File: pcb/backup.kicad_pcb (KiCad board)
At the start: 2 copper layers, 47.6 x 63.5 mm, 44 parts, among them CON1 BARREL_JACK, IC1 ATMEGA168A-P, P1 CONN_02X02, P2 CONN_01X06, P3 CONN_01X07, P4 CONN_01X04, P5 CONN_01X07, SW1 SW_PUSH, U1 MAX6817, U2 LM7805CT, U3 MIC94090, Y1 Crystal

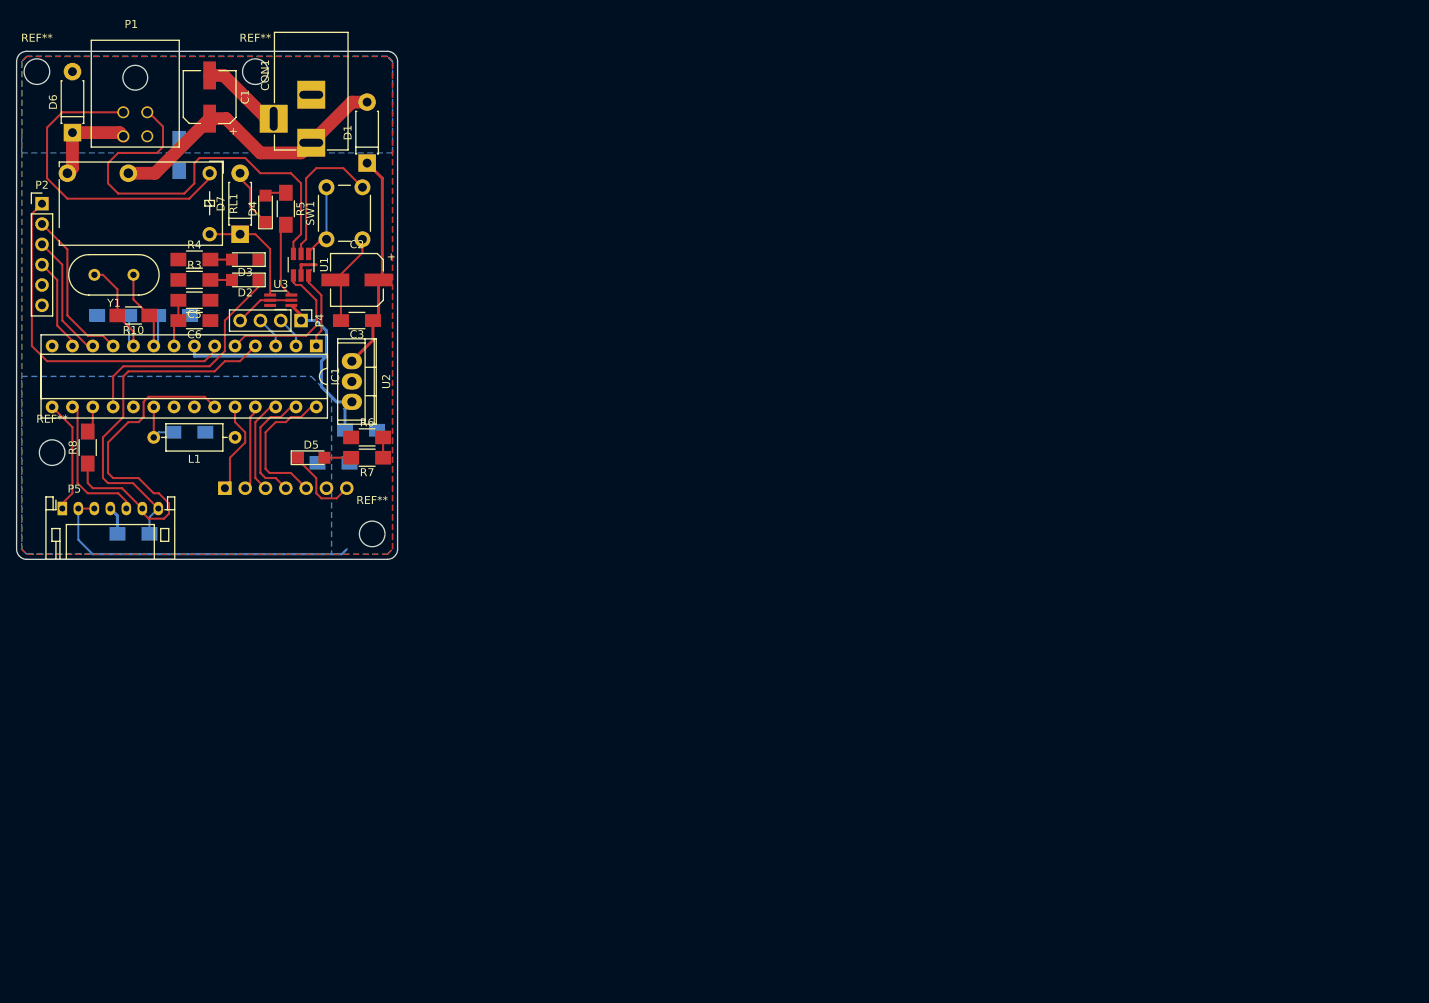
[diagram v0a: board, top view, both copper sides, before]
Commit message: wip
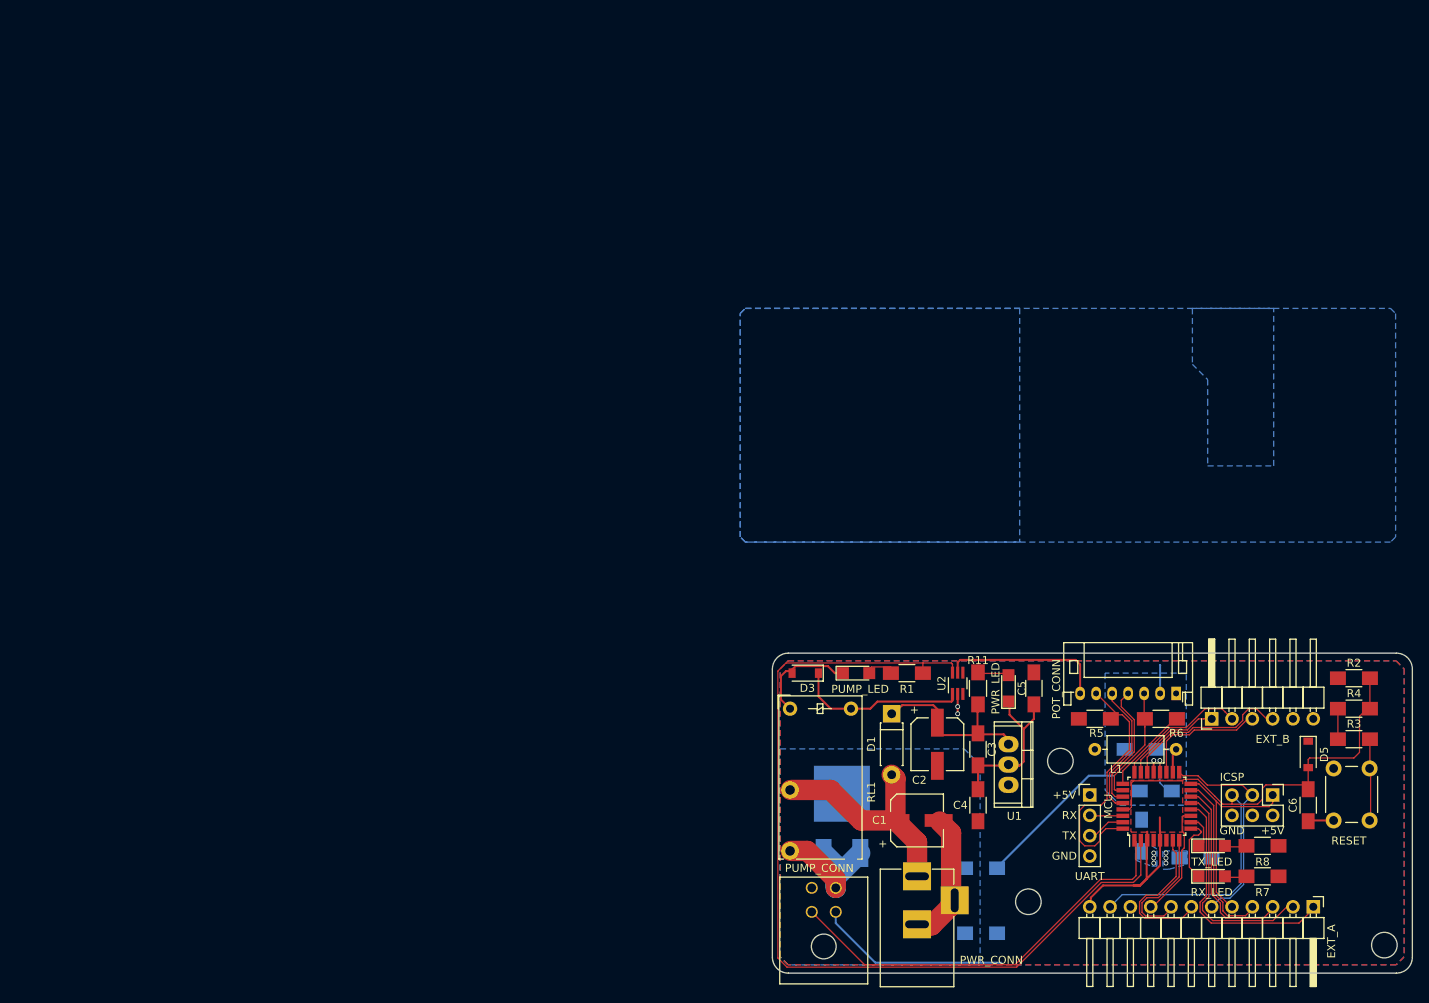
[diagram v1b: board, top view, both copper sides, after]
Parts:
- removed C8: 22pF, Capacitors_SMD:C_1206_HandSoldering
- removed CON1: BARREL_JACK, Connect:BARREL_JACK
- removed D4: LED, LEDs:LED_1206
- removed D6, D7: D, Diodes_ThroughHole:D_DO-41_SOD81_P7.62mm_Horizontal
- removed IC1: ATMEGA168A-P, Housings_DIP:DIP-28_W7.62mm_Socket
- removed P1: CONN_02X02, Connectors_Molex:Molex_Microfit3_Header_02x02_Angled_43045-040x
- removed P2: CONN_01X06, Pin_Headers:Pin_Header_Straight_1x06_Pitch2.54mm
- removed P3: CONN_01X07, Pin_Headers:Pin_Header_Angled_1x07_Pitch2.54mm
- removed P4: CONN_01X04, Pin_Headers:Pin_Header_Straight_1x04_Pitch2.54mm
- removed P5: CONN_01X07, Connectors_JST:JST_PH_S7B-PH-K_07x2.00mm_Angled
- removed the REF** at (114.0, 96.1)
- removed the REF** at (74.0, 86.0)
- removed the REF** at (72.1, 38.4)
- removed the REF** at (99.4, 38.4)
- removed SW1: SW_PUSH, Buttons_Switches_ThroughHole:SW_PUSH_6mm
- removed U3: MIC94090, TO_SOT_Packages_SMD:SOT-363_SC-70-6_Handsoldering
- removed Y1: Crystal, Crystals:Crystal_HC49-U_Vertical
- added C11: 100nF, Capacitors_SMD:C_1206_HandSoldering, B.Cu at (210.1, 123.1)
- added C12: 10nF, Capacitors_SMD:C_1206_HandSoldering, B.Cu at (212.0, 128.3)
- added EXT_A: CONN_01X12, Pin_Headers:Pin_Header_Angled_1x12_Pitch2.54mm, F.Cu at (231.6, 142.7)
- added EXT_B: CONN_01X06, Pin_Headers:Pin_Header_Angled_1x06_Pitch2.54mm, F.Cu at (218.9, 119.3)
- added ICSP: CONN_02X03, Pin_Headers:Pin_Header_Straight_2x03_Pitch2.54mm, F.Cu at (226.6, 128.8)
- added MCU: ATMEGA168-20AU, Housings_QFP:TQFP-32_7x7mm_Pitch0.8mm, F.Cu at (212.1, 130.2)
- added POT_CONN: CONN_01X07, Connectors_JST:JST_PH_S7B-PH-K_07x2.00mm_Angled, F.Cu at (214.5, 116.1)
- added PUMP_CONN: CONN_02X02, Connectors_Molex:Molex_Microfit3_Header_02x02_Angled_43045-040x, F.Cu at (172.0, 143.4)
- added PUMP_LED: PUMP_LED, LEDs:LED_1206, F.Cu at (174.5, 113.5)
- added PWR_CONN: BARREL_JACK, Connectors:BARREL_JACK, F.Cu at (182.1, 138.9)
- added PWR_LED: PWR_LED, LEDs:LED_1206, F.Cu at (193.5, 115.4)
- added R11: 1.5K, Resistors_SMD:R_1206_HandSoldering, F.Cu at (189.7, 115.4)
- added REF**: MountingHole_3.2mm_M3, Mounting_Holes:MountingHole_3.2mm_M3, F.Cu at (200.0, 124.5)
- added REF**: MountingHole_3.2mm_M3, Mounting_Holes:MountingHole_3.2mm_M3, F.Cu at (240.5, 147.5)
- added REF**: MountingHole_3.2mm_M3, Mounting_Holes:MountingHole_3.2mm_M3, F.Cu at (196.0, 142.1)
- added RESET: SW_PUSH, Buttons_Switches_THT:SW_PUSH_6mm, F.Cu at (234.2, 132.0)
- added RX_LED: RX_LED, LEDs:LED_1206, F.Cu at (218.9, 138.9)
- added TX_LED: TX_LED, LEDs:LED_1206, F.Cu at (218.9, 135.1)
- added UART: CONN_01X04, Pin_Headers:Pin_Header_Straight_1x04_Pitch2.54mm, F.Cu at (203.7, 128.8)
- C4: moved to F.Cu
- C6: value 10nF -> 100nF
- C9: value 22pF -> 100nF
- D1: footprint Diodes_ThroughHole:D_DO-41_SOD81_P7.62mm_Horizontal -> Diodes_THT:D_DO-41_SOD81_P7.62mm_Horizontal
- D2: value LED -> D_Schottky; footprint LEDs:LED_1206 -> TO_SOT_Packages_SMD:TO-252-2_Rectifier; moved to B.Cu
- D3, D5: value LED -> D_Schottky; footprint LEDs:LED_1206 -> Diodes_SMD:D_SOD-123
- R1: value 0 -> 1.5k; moved to F.Cu
- R10: value 1M -> 0; moved to B.Cu
- R2: value 0 -> 4k7; moved to F.Cu
- R3, R4: value 150R -> 150
- R5: value 1.5k -> 100k
- R6: value 150R -> 10k
- R8: value 10k -> 150R
- R9: value 100k -> 0
- RL1: footprint Relays_ThroughHole:Relay_SPST_Finder_32.21-x300 -> Relays_THT:Relay_SPST_Finder_32.21-x300
- U1: value MAX6817 -> LM7805CT; footprint TO_SOT_Packages_SMD:SOT-23-6_Handsoldering -> Power_Integrations:TO-220
- U2: value LM7805CT -> MIC94090; footprint Power_Integrations:TO-220 -> TO_SOT_Packages_SMD:SOT-363_SC-70-6_Handsoldering
- moved R3 155.9 mm to (236.7, 121.8), turned to 180 degrees
- moved R4 155.4 mm to (236.7, 118.0)
- moved R8 155.1 mm to (225.3, 135.1), turned to 180 degrees
- moved C6 151.8 mm to (231.0, 130.0), turned to 270 degrees
- moved C9 144.1 mm to (210.2, 133.9), turned to 90 degrees
- moved C7 136.6 mm to (216.9, 136.7)
- moved R2 130.4 mm to (236.7, 114.2), turned to 180 degrees
- moved D5 130.0 mm to (231.0, 123.7), turned to 270 degrees
- moved R10 126.5 mm to (190.1, 137.9)
- moved C1 126.5 mm to (182.1, 132.0), turned to 0 degrees
- moved R7 123.5 mm to (225.3, 138.9)
- moved R5 119.5 mm to (204.3, 119.3), turned to 0 degrees
- moved R9 117.1 mm to (190.1, 146.1)
- moved C5 115.6 mm to (196.7, 115.4), turned to 270 degrees
- moved L1 114.3 mm to (204.3, 123.1), turned to 0 degrees
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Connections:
- C2 pad 1: /REG_PWR -> REG_PWR
- C3 pad 1: /REG_PWR -> REG_PWR
- C6 pad 1: Vcc -> ~RESET
- C7 pad 1: AVcc -> Vcc
- C7 pad 2: AVss -> GND
- C9 pad 1: GND -> Vcc
- C9 pad 2: /XTAL2 -> GND
- D1 pad 1: /REG_PWR -> REG_PWR
- D2 pad 1: RX_LED -> /PUMP+
- D2 pad 2: Net-(D2-Pad2) -> PGND
- D3 pad 1: TX_LED -> /COIL_PWR
- D3 pad 2: Net-(D3-Pad2) -> GND
- D5 pad 1: GND -> Vcc
- D5 pad 2: Net-(D5-Pad2) -> ~RESET
- R1 pad 1: PGND -> Net-(D4-Pad2)
- R1 pad 2: GND -> PUMP
- R10 pad 1: /XTAL1 -> AVss
- R10 pad 2: /XTAL2 -> PGND
- R2 pad 1: AVss -> ~RESET
- R2 pad 2: GND -> Vcc
- R3 pad 1: Vcc -> Net-(R3-Pad1)
- R3 pad 2: Net-(D2-Pad2) -> Net-(R3-Pad2)
- R4 pad 1: Vcc -> Net-(R3-Pad2)
- R4 pad 2: Net-(D3-Pad2) -> ~RESET
- R5 pad 1: Net-(D4-Pad2) -> Vcc
- R5 pad 2: PUMP -> ~OVRFLW
- R6 pad 1: Vcc -> MOISTURE
- R6 pad 2: Net-(R6-Pad2) -> MOIST+
- R7 pad 1: Net-(R6-Pad2) -> Vcc
- R7 pad 2: Net-(D5-Pad2) -> Net-(D6-Pad2)
- R8 pad 1: MOISTURE -> Vcc
- R8 pad 2: /MOIST+ -> Net-(D7-Pad2)
- R9 pad 1: Vcc -> PGND
- R9 pad 2: ~OVRFLW -> GND
- U1 pad 1: Net-(SW1-Pad1) -> REG_PWR
- U1 pad 3: /LVL_SWTCH -> Vcc
- U2 pad 1: /REG_PWR -> /COIL_PWR
- U2 pad 3: Vcc -> Net-(U2-Pad3)
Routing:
- net PUMP: track 9.64 -> 116.3 mm
- net ~RESET: track 0.00 -> 81.7 mm
- net /LVL_SWTCH: track 54.0 -> 0.00 mm
- net ~LEVEL_ALERT: track 0.00 -> 52.8 mm
- net Vcc: track 46.7 -> 2.20 mm
- net /EXT_B1: track 43.1 -> 0.00 mm
- net MOISTURE: track 46.6 -> 14.7 mm
- net EXT_D0: track 0.00 -> 30.1 mm
- net SCK: track 0.00 -> 28.6 mm
- net GND: track 142.7 -> 114.4 mm, vias 0 -> 2
- net EXT_D1: track 0.00 -> 27.6 mm
- net /REG_PWR: track 27.1 -> 0.00 mm
- net MISO: track 0.00 -> 26.8 mm
- net EXT_D2: track 0.00 -> 24.1 mm
- net MOSI: track 0.00 -> 22.5 mm
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- added copper zone on F.Cu, net GND
- added copper zone on B.Cu, net Vcc
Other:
- board size 47.6 x 63.5 mm -> 80 x 40 mm
- net class 12V: clearance 0.7 -> 0.254; trace_width 1.6 -> 2.54; via_dia 6 -> 0.6; via_drill 5 -> 0.4
- net class 5V added: clearance 0.1524, trace_width 0.254, via_dia 0.6, via_drill 0.4
- net class Default: clearance 0.254 -> 0.1524; trace_width 0.254 -> 0.1524
- net class Power removed
- rule trace_clearance: 0.254 -> 0.1524
- rule trace_min: 0.254 -> 0.1524
- board text added: "+5V"
- board text added: "GND"
- board text added: "RX"
- board text added: "TX"
